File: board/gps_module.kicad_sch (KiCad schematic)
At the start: 16 parts, among them IC1 RT9193-33GB, IC2 NJG1130KA1-TE1, J5 Conn_Coaxial, U6 NEO-M7N

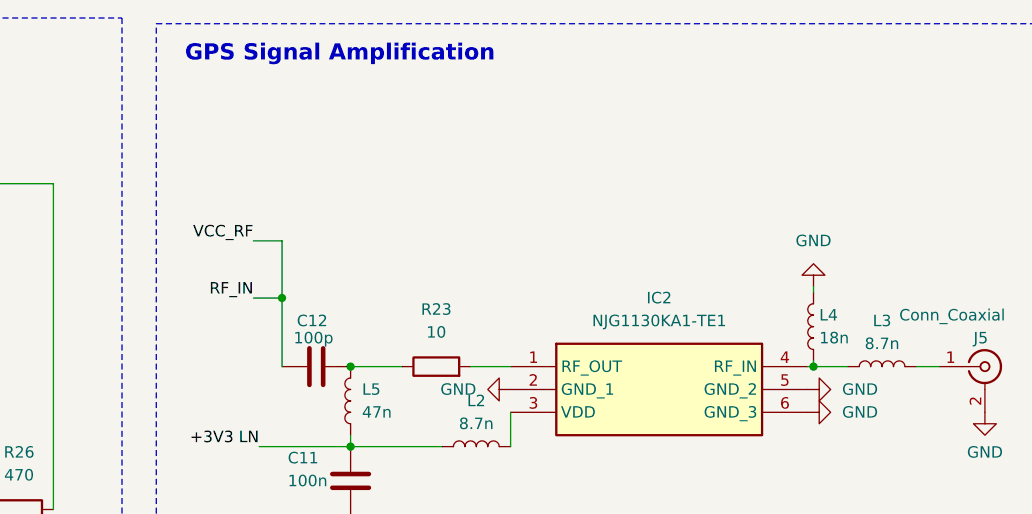
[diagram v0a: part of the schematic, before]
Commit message: Minor improvement to the board
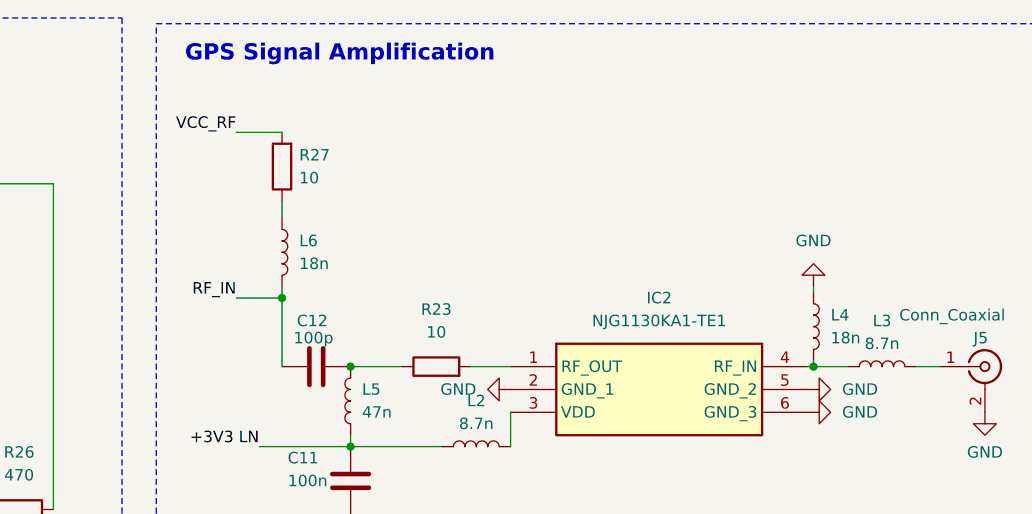
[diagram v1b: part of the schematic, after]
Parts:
- added L6: 18n, Inductor_SMD:L_0805_2012Metric, symbol Device:L
- added R27: 10, Resistor_SMD:R_0603_1608Metric, symbol Device:R
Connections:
- net GND: now also L4.1; no longer L4.2
- net RF_IN: now also L6.2; no longer U6.9 (VCC_RF)
- net at IC2.4 (RF_IN), L3.1: now also L4.2; no longer L4.1
- new net: L6.1, R27.1
- new net VCC_RF: R27.2, U6.9 (VCC_RF)
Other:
- moved on the sheet: L4
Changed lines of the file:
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@@
     (rev "1.0")
   )
+  (junction (at 199.39 100.33) (diameter 0) (color 0 0 0 0)
+  )
+  (junction (at 199.39 109.22) (diameter 0) (color 0 0 0 0)
+  )
+  (junction (at 78.74 101.6) (diameter 0) (color 0 0 0 0)
+  )
+  (junction (at 250.825 100.33) (diameter 0) (color 0 0 0 0)
+  )
+  (junction (at 128.27 76.2) (diameter 0) (color 0 0 0 0)
+  )
+  (junction (at 27.94 99.06) (diameter 0) (color 0 0 0 0)
+  )
   (junction (at 191.77 92.71) (diameter 0) (color 0 0 0 0)
-  )
-  (junction (at 199.39 100.33) (diameter 0) (color 0 0 0 0)
-  )
-  (junction (at 199.39 109.22) (diameter 0) (color 0 0 0 0)
-  )
-  (junction (at 78.74 101.6) (diameter 0) (color 0 0 0 0)
-  )
-  (junction (at 250.825 100.33) (diameter 0) (color 0 0 0 0)
-  )
-  (junction (at 128.27 76.2) (diameter 0) (color 0 0 0 0)
-  )
-  (junction (at 27.94 99.06) (diameter 0) (color 0 0 0 0)
   )
   (junction (at 69.215 91.44) (diameter 0) (color 0 0 0 0)
@@
   (no_connect (at 115.57 95.885))
   (no_connect (at 115.57 93.345))
-  (wire (pts (xy 188.595 92.71) (xy 191.77 92.71))
+  (wire (pts (xy 186.69 92.71) (xy 191.77 92.71))
+    (stroke (width 0) (type default))
+  )
+  (wire (pts (xy 191.77 92.71) (xy 191.77 100.33))
     (stroke (width 0) (type default))
   )
@@
     (stroke (width 0) (type default))
   )
-  (wire (pts (xy 191.77 92.71) (xy 191.77 100.33))
+  (wire (pts (xy 191.77 81.915) (xy 191.77 83.82))
     (stroke (width 0) (type default))
   )
@@
     (stroke (width 0) (type default))
   )
-  (wire (pts (xy 191.77 86.36) (xy 188.595 86.36))
+  (wire (pts (xy 186.69 74.295) (xy 191.77 74.295))
     (stroke (width 0) (type default))
   )
@@
     (stroke (width 0) (type default))
   )
-  (wire (pts (xy 191.77 86.36) (xy 191.77 92.71))
+  (wire (pts (xy 191.77 91.44) (xy 191.77 92.71))
     (stroke (width 0) (type default))
   )
@@
     (effects (font (size 1.27 1.27)) (justify left bottom))
   )
-  (label "RF_IN" (at 188.595 92.71 180) (fields_autoplaced)
+  (label "RF_IN" (at 186.69 92.71 180) (fields_autoplaced)
     (effects (font (size 1.27 1.27)) (justify right bottom))
   )
@@
     (effects (font (size 1.27 1.27)) (justify left bottom))
   )
-  (label "VCC_RF" (at 188.595 86.36 180) (fields_autoplaced)
+  (label "VCC_RF" (at 186.69 74.295 180) (fields_autoplaced)
     (effects (font (size 1.27 1.27)) (justify right bottom))
   )
@@
     )
   )
+  (symbol (lib_id "Device:R") (at 191.77 78.105 180) (unit 1)
+    (in_bom yes) (on_board yes) (dnp no) (fields_autoplaced)
+    (property "Reference" "R27" (at 193.675 76.835 0)
+      (effects (font (size 1.27 1.27)) (justify right))
+    )
+    (property "Value" "10" (at 193.675 79.375 0)
+      (effects (font (size 1.27 1.27)) (justify right))
+    )
+    (property "Footprint" "Resistor_SMD:R_0603_1608Metric" (at 193.548 78.105 90)
+      (effects (font (size 1.27 1.27)) hide)
+    )
+    (property "Datasheet" "~" (at 191.77 78.105 0)
+      (effects (font (size 1.27 1.27)) hide)
+    )
+    (pin "1")
+    (pin "2")
+    (instances
+      (project "uav_project"
+        (path "/a8bf0924-b264-4c19-8c7e-9c0e131cacba/cca59cde-6ab1-4762-8541-6f874c4d6e1b"
+          (reference "R27") (unit 1)
+        )
+      )
+    )
+  )
   (symbol (lib_id "Device:C") (at 69.215 95.25 0) (unit 1)
     (in_bom yes) (on_board yes) (dnp no)
@@
     )
   )
-  (symbol (lib_id "Device:L") (at 250.825 95.885 180) (unit 1)
-    (in_bom yes) (on_board yes) (dnp no) (fields_autoplaced)
-    (property "Reference" "L4" (at 251.46 94.615 0)
-      (effects (font (size 1.27 1.27)) (justify right))
-    )
-    (property "Value" "18n" (at 251.46 97.155 0)
-      (effects (font (size 1.27 1.27)) (justify right))
+  (symbol (lib_id "Device:L") (at 250.825 95.885 0) (unit 1)
+    (in_bom yes) (on_board yes) (dnp no) (fields_autoplaced)
+    (property "Reference" "L4" (at 252.73 94.615 0)
+      (effects (font (size 1.27 1.27)) (justify left))
+    )
+    (property "Value" "18n" (at 252.73 97.155 0)
+      (effects (font (size 1.27 1.27)) (justify left))
     )
     (property "Footprint" "Inductor_SMD:L_0805_2012Metric" (at 250.825 95.885 0)
@@
         )
       )
+    )
+  )
+  (symbol (lib_id "Device:L") (at 191.77 87.63 0) (unit 1)
+    (in_bom yes) (on_board yes) (dnp no) (fields_autoplaced)
+    (property "Reference" "L6" (at 193.675 86.36 0)
+      (effects (font (size 1.27 1.27)) (justify left))
+    )
+    (property "Value" "18n" (at 193.675 88.9 0)
+      (effects (font (size 1.27 1.27)) (justify left))
+    )
+    (property "Footprint" "Inductor_SMD:L_0805_2012Metric" (at 191.77 87.63 0)
+      (effects (font (size 1.27 1.27)) hide)
+    )
+    (property "Datasheet" "~" (at 191.77 87.63 0)
+      (effects (font (size 1.27 1.27)) hide)
+    )
+    (pin "1")
+    (pin "2")
+    (instances
+      (project "uav_project"
+        (path "/a8bf0924-b264-4c19-8c7e-9c0e131cacba/cca59cde-6ab1-4762-8541-6f874c4d6e1b"
+          (reference "L6") (unit 1)
+        )
+      )
